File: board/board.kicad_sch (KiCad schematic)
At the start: 34 parts

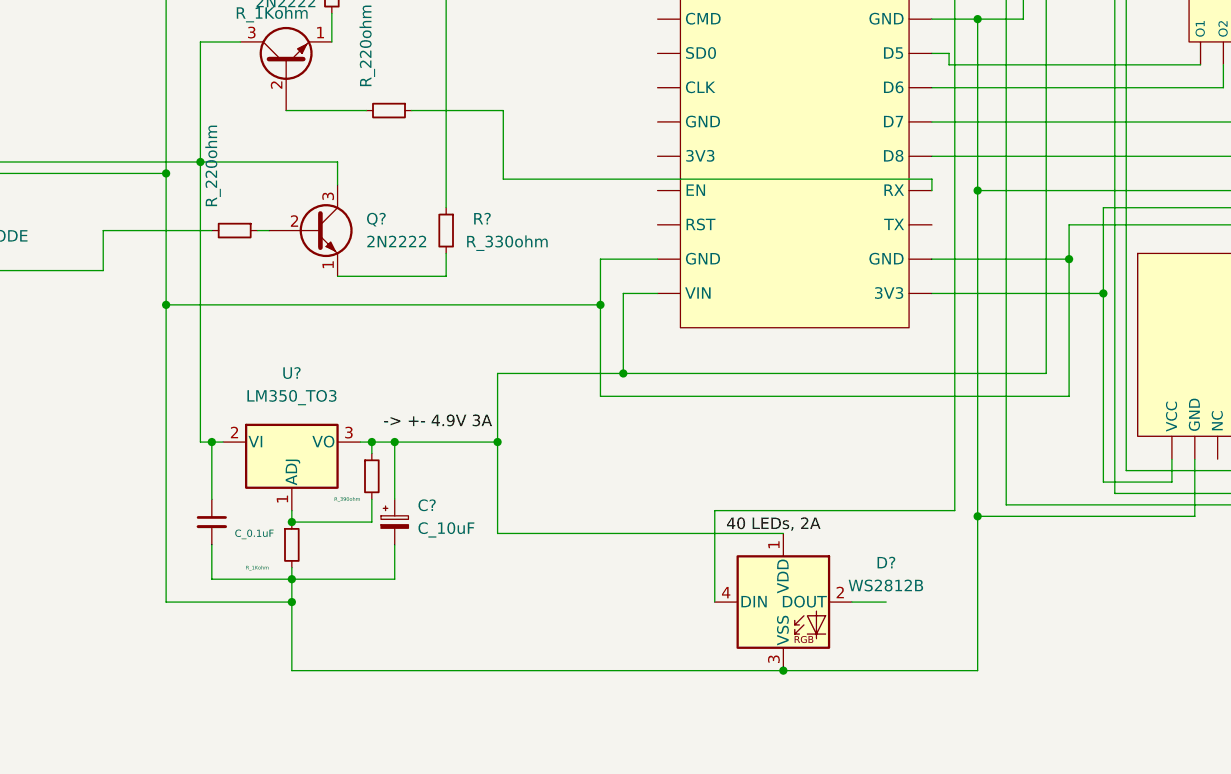
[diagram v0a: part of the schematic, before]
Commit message: .
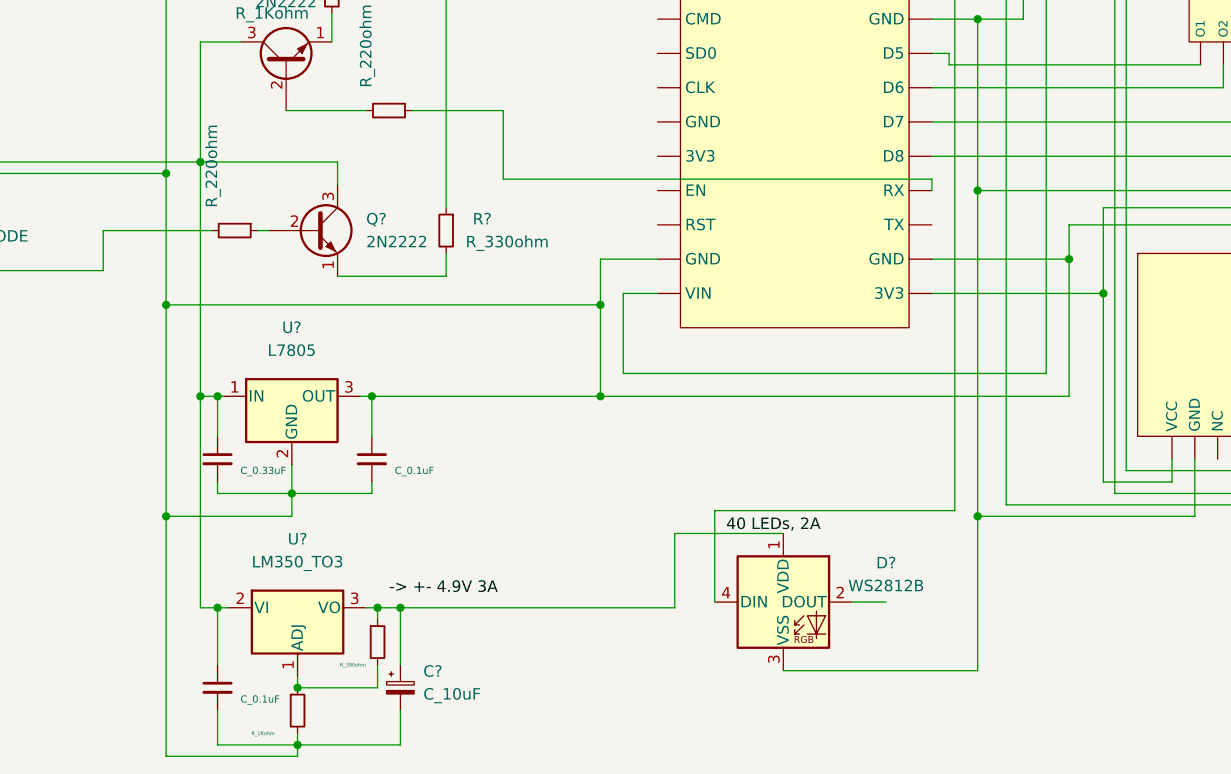
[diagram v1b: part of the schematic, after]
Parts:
- added C?: C_0.1uF, symbol Device:C_Small
- added C?: C_0.33uF, symbol Device:C_Small
- added U?: L7805, symbol Regulator_Linear:L7805
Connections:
- net 40 LEDs, 2A: no longer U?. (VIN), U?.8 (VCC)
- net at U?. (VIN): now also R?.1; no longer U?. (VCC)
- net at -?. (load-), C?.1, D?.2 (A)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: now also C?.1, U?.1 (IN)
- net at U?. (VCC): now also U?. (VIN)
- new net: -?. (load-), BT?.2 (-), C?.1, C?.2, C?.2, C?.2, C?.2, J?.5 (GND), R?.1, R?.2, U?. (VIN), U?.2 (GND), U?.3 (OUT), U?.4 (GND)
- new net: U?. (VIN), U?.8 (VCC)
- new net: -?.1 (A0), -?.2 (A1), -?.3 (A2), -?.4 (GND), -?.7 (WP), D?.3 (VSS), U?. (VCC), U?. (VCC), U?. (VIN)
- new net: U?. (VCC), U?. (VCC), U?. (VIN)
- new net: U?. (VCC), U?. (VIN) (x3)
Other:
- moved on the sheet: C?, U?

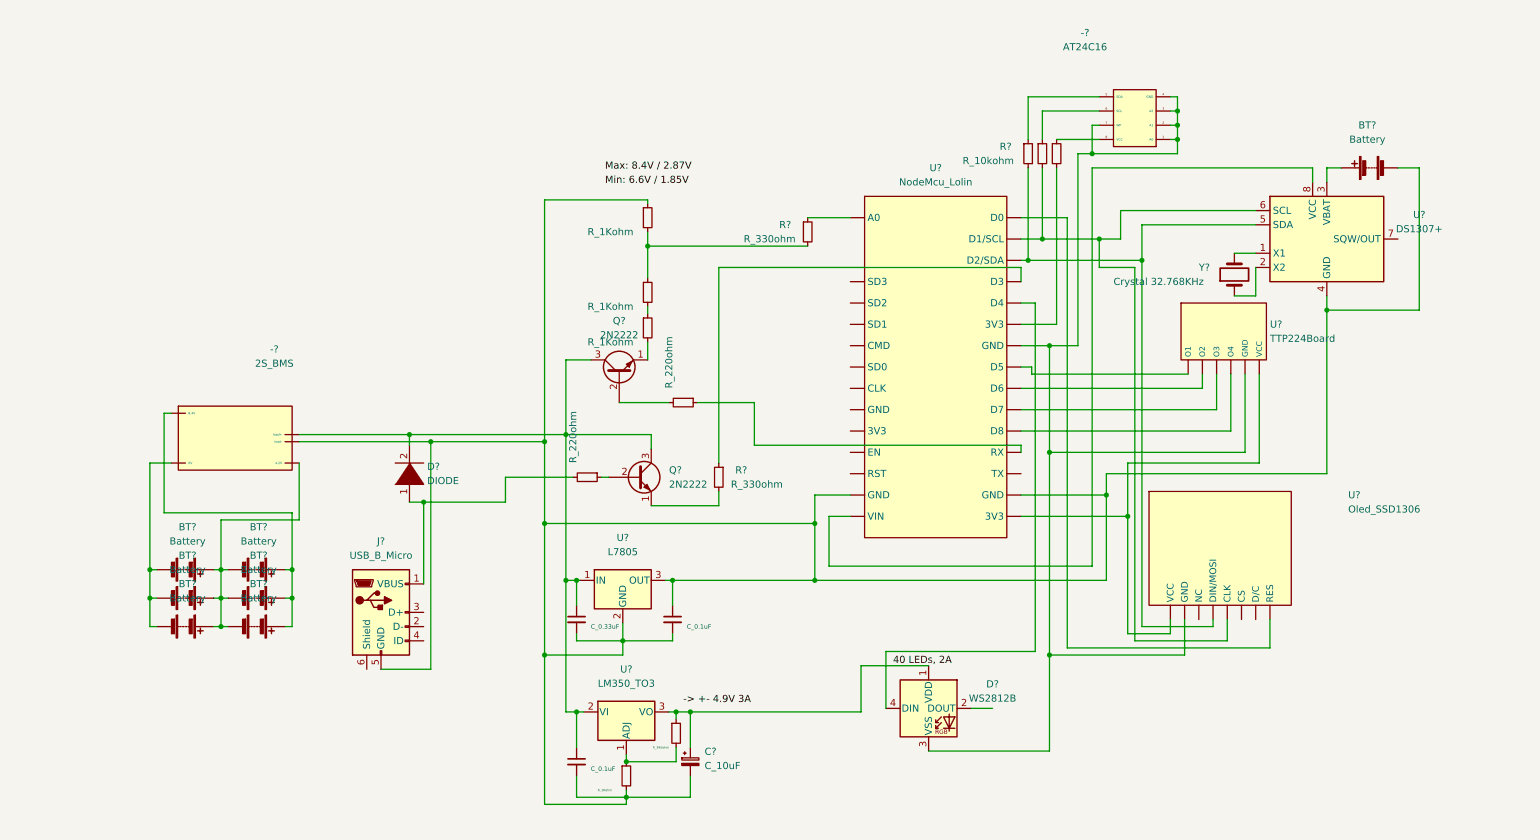
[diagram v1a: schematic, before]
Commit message: edit
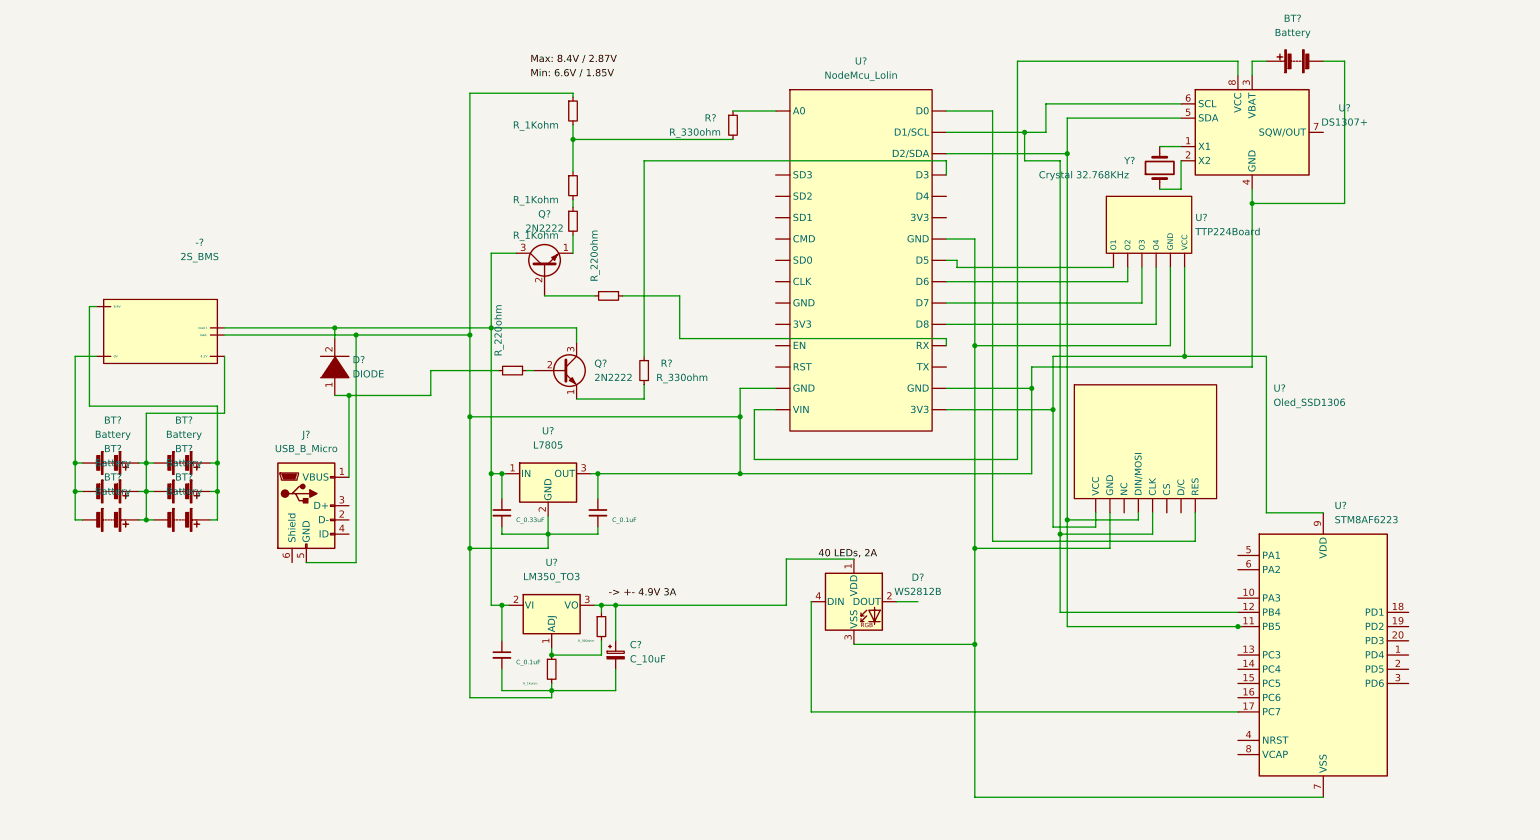
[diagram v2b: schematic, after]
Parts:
- removed -?: AT24C16, symbol custom_boards:AT24C16
- removed R? (x3): R_10kohm, symbol Device:R_Small
- added U?: STM8AF6223, Package_SO:TSSOP-20_4.4x6.5mm_P0.65mm, symbol MCU_ST_STM8:STM8AF6223
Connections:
- net at U?. (VIN): now also R?.1; no longer U?. (VCC)
- net at D?.4 (DIN): now also U?.17 (PC7); no longer U?. (VIN)
- net at U?. (VCC): now also U?. (VIN)
- new net: U?. (VCC), U?. (VIN), U?.11 (PB5), U?.5 (SDA)
- new net: U?. (VCC), U?. (VIN), U?.12 (PB4), U?.6 (SCL)
- new net: D?.3 (VSS), U?. (VCC), U?. (VCC), U?. (VIN), U?.7 (VSS)
- new net: U?. (VCC), U?. (VCC), U?. (VIN), U?.9 (VDD)
- new net: U?. (VCC), U?. (VIN) (x3)
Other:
- moved on the sheet: -?, BT?, C?, D?, J?, Q?, R?, U?, Y?

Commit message: a chnage
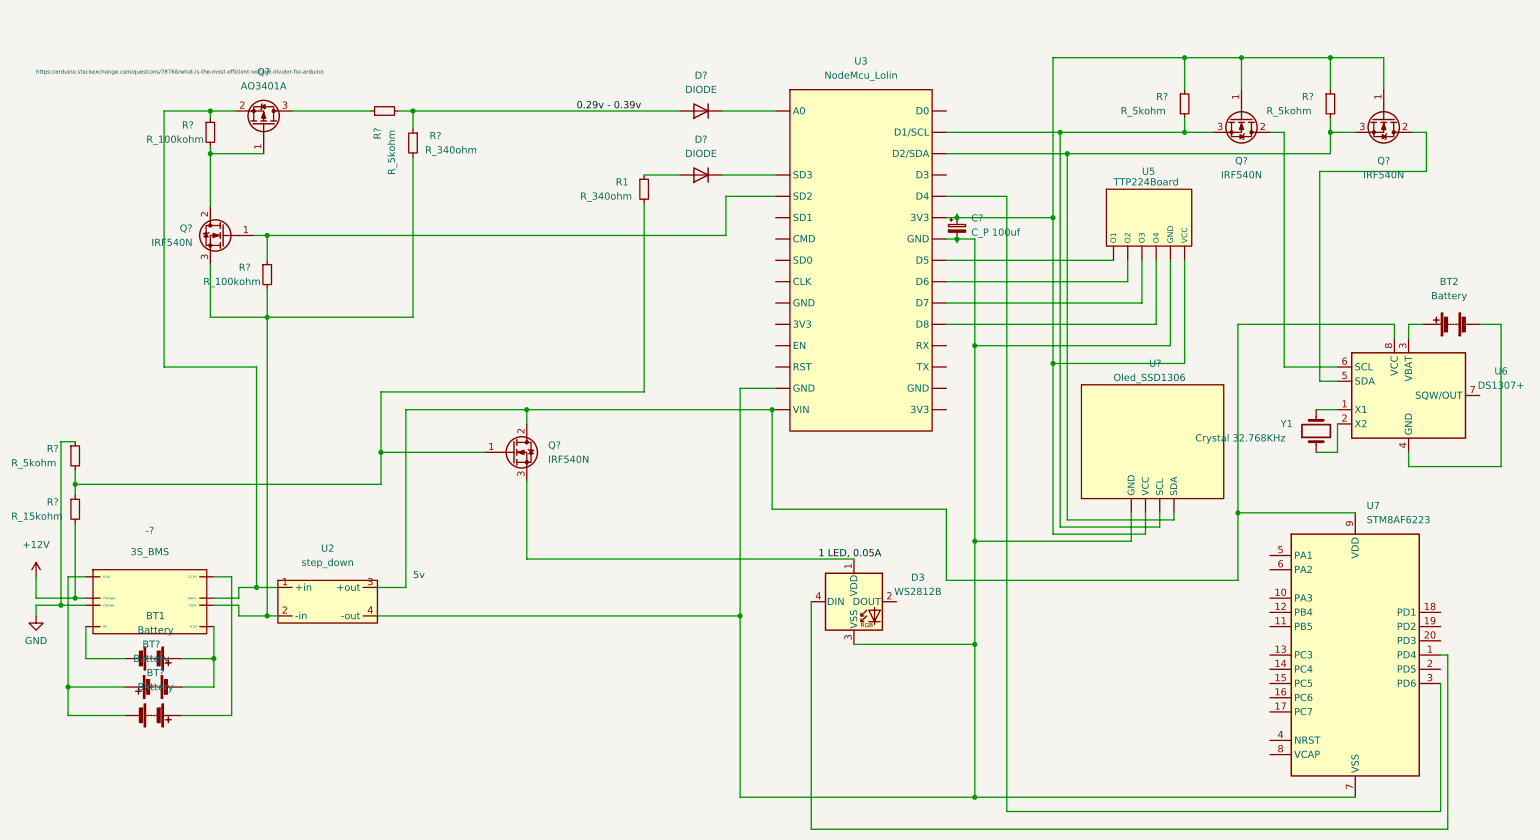
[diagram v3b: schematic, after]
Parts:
- removed -?: 2S_BMS, symbol custom_boards:2S_BMS
- removed BT? (x5): Battery, symbol Device:Battery
- removed C? (x2): C_0.1uF, symbol Device:C_Small
- removed C?: C_10uF, symbol Device:C_Polarized_Small
- removed C?: C_0.33uF, symbol Device:C_Small
- removed D?: DIODE, symbol pspice:DIODE
- removed J?: USB_B_Micro, symbol Connector:USB_B_Micro
- removed Q? (x2): 2N2222, Package_TO_SOT_THT:TO-39-3, symbol custom_boards:2N2222
- removed R? (x2): R_220ohm, symbol Device:R_Small
- removed R?: R_390ohm, symbol Device:R_Small
- removed R? (x2): R_330ohm, symbol Device:R_Small
- removed R? (x4): R_1Kohm, symbol Device:R_Small
- removed U?: L7805, symbol Regulator_Linear:L7805
- removed U?: Oled_SSD1306, symbol custom_boards:Oled_SSD1306
- removed U?: LM350_TO3, Package_TO_SOT_THT:TO-3, symbol Regulator_Linear:LM350_TO3
- added -?: 3S_BMS, symbol custom_boards:3S_BMS
- added BT? (x2): Battery, symbol Device:Battery
- added C?: C_P 100uf, symbol Device:C_Polarized_Small
- added D? (x2): DIODE, symbol Simulation_SPICE:DIODE
- added Q? (x4): IRF540N, Package_TO_SOT_THT:TO-220-3_Vertical, symbol Transistor_FET:IRF540N
- added Q?: AO3401A, Package_TO_SOT_SMD:SOT-23, symbol Transistor_FET:AO3401A
- added R1, R?: R_340ohm, symbol Device:R_Small
- added R? (x2): R_100kohm, symbol Device:R_Small
- added R? (x4): R_5kohm, symbol Device:R_Small
- added R?: R_15kohm, symbol Device:R_Small
- added U2: step_down, symbol custom_boards:step_down
- added U?: Oled_SSD1306, symbol custom_boards:Oled_SSD1306
- gave numbers to parts that had none: 8
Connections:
- net at BT2.2 (-), U6.4 (GND): no longer U3. (VIN)
- net at U3. (VIN), U6.8 (VCC): now also U7.9 (VDD), Q?.2 (D), U2.3 (+out)
- net at BT1.1 (+): now also -?. (load-), BT?.2 (-)
- net at BT1.2 (-): now also -?. (load-)
- net at D3.3 (VSS), U3. (VIN), U5. (VCC)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: now also C?.2, U2.4 (-out), U?. (VCC)
- net at U3. (VIN), U5. (VCC): now also C?.1, Q?.1 (G), Q?.1 (G), R?.1, R?.1, U?. (VCC)
- net at U3. (VIN): now also Q?.3 (S), R?.2, U?. (VCC); no longer U5. (VCC)
- net at D3.4 (DIN): now also U7.1 (PD4); no longer U7.17 (PC7)
- net at U7.3 (PD6): now also U3. (VIN)
- net 40 LEDs, 2A renamed 1 LED, 0.05A
- net 1 LED, 0.05A: now also Q?.3 (S)
- new net: Q?.2 (D), U6.5 (SDA)
- new net: Q?.2 (D), U6.6 (SCL)
- new net: D?.1 (A), R1.1
- new net: Q?.1 (G), R1.2, R?.1, R?.2
- new net: Q?.1 (G), R?.1, U3. (VIN)
- new net: Q?.1 (G), Q?.2 (D), R?.2
- new net: -?. (load-), Q?.3 (S), R?.2, R?.2, U2.2 (-in)
- new net: U3. (VIN), U5. (VCC) (x4)
- new net: -?. (load-), Q?.2 (S), R?.1, U2.1 (+in)
- new net: Q?.3 (D), R?.1
- new net: D?.2 (K), U3. (VIN) (x2)
- new net: -?. (load-), BT?.1 (+)
- new net: -?. (load-), BT?.1 (+), BT?.2 (-)
- new net: Q?.3 (S), R?.2, U3. (VIN), U?. (VCC)
- new net +12V: -?. (load-), R?.2
- new net 0.29v - 0.39v: D?.1 (A), R?.1, R?.2
- new net GND: -?. (load-), R?.1
- now unconnected: U7.11 (PB5), U7.12 (PB4)
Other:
- note added: "5v"
- note added: "https://arduino.stackexchange.com/questions/78768/what-is-the-most-efficient-voltage-divider-for-arduino"
- moved on the sheet: BT1, BT2, U5, U6, U7, Y1
